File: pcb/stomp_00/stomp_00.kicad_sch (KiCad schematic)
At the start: 4 parts, among them U1 Teensy4.1, U2 74HC595, U5 74HC165, U7 74HC4051

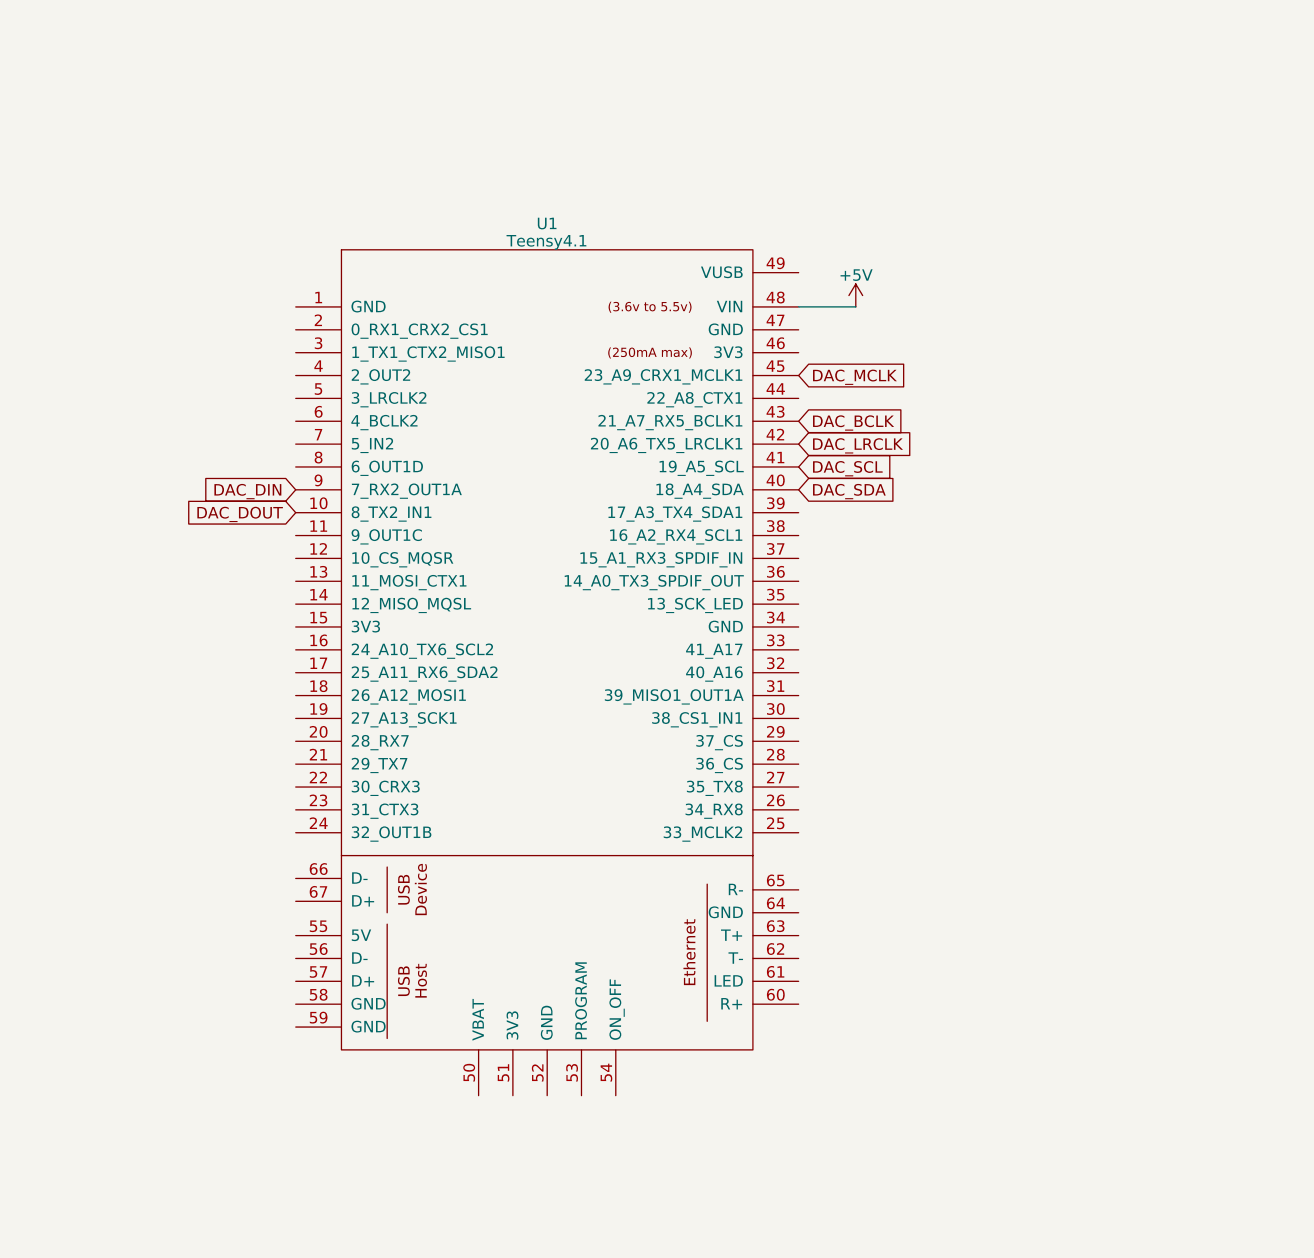
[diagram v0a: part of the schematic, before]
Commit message: came back to the project
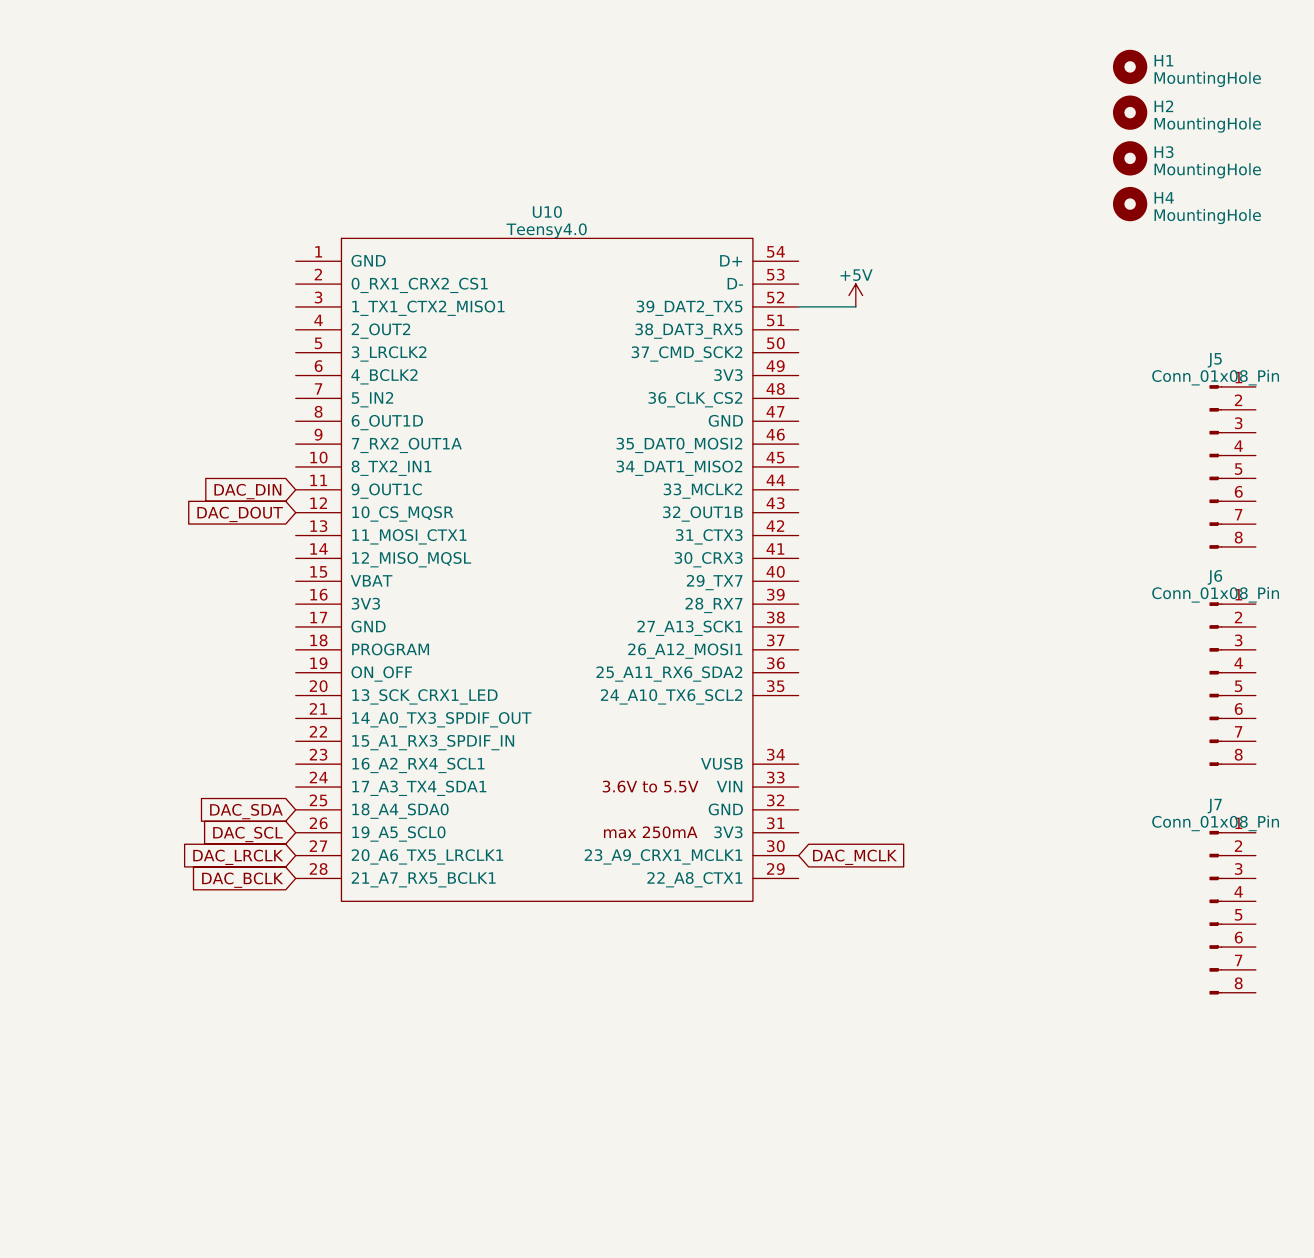
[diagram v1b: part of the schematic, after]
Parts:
- removed U1: Teensy4.1, symbol teensy:Teensy4.1
- added H1, H2, H3, H4: MountingHole, MountingHole:MountingHole_3.2mm_M3, symbol Mechanical:MountingHole
- added J5, J6, J7: Conn_01x08_Pin, Connector_PinHeader_2.54mm:PinHeader_1x08_P2.54mm_Vertical, symbol Connector:Conn_01x08_Pin
- added U10: Teensy4.0, symbol teensy:Teensy4.0
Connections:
- net +5V: now also U10.52 (39_DAT2_TX5)
- net DAC_BCLK: now also U10.28 (21_A7_RX5_BCLK1)
- net DAC_DIN: now also U10.11 (9_OUT1C)
- net DAC_DOUT: now also U10.12 (10_CS_MQSR)
- net DAC_LRCLK: now also U10.27 (20_A6_TX5_LRCLK1)
- net DAC_MCLK: now also U10.30 (23_A9_CRX1_MCLK1)
- net DAC_SCL: now also U10.26 (19_A5_SCL0)
- net DAC_SDA: now also U10.25 (18_A4_SDA0)
